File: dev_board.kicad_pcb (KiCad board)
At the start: 2 copper layers, 60 x 70 mm, 148 parts, among them IC1 AD9609BCPZRL7-80, IC2 ENS161-BLGT_LGA9_T&R_1k5, IC3 ICM-42670-P, IC4 IWRL6432BDBAAMFR, IC5 MP4541GN-Z, IC6 THS8136IPHPR, IC7 TPS40304ADRCR, IC8 XCC1352R1F3RGZR, J2 Conn_02x26_Odd_Even, J4 SM03B-SRSS-TB, J5 STM32H7 GPIO/Fabric Breakout A, J6 STM32H7 GPIO/Fabric Breakout B, J9 HS/IWRL Fabric Breakout, SW1 SW_Push, SW2 SW_Push, U1 RP2350_80QFN, U2 LPS22HH, U3 STM32H750VBTx, U4 LAN8742A, Y1 ABM8-272-T3

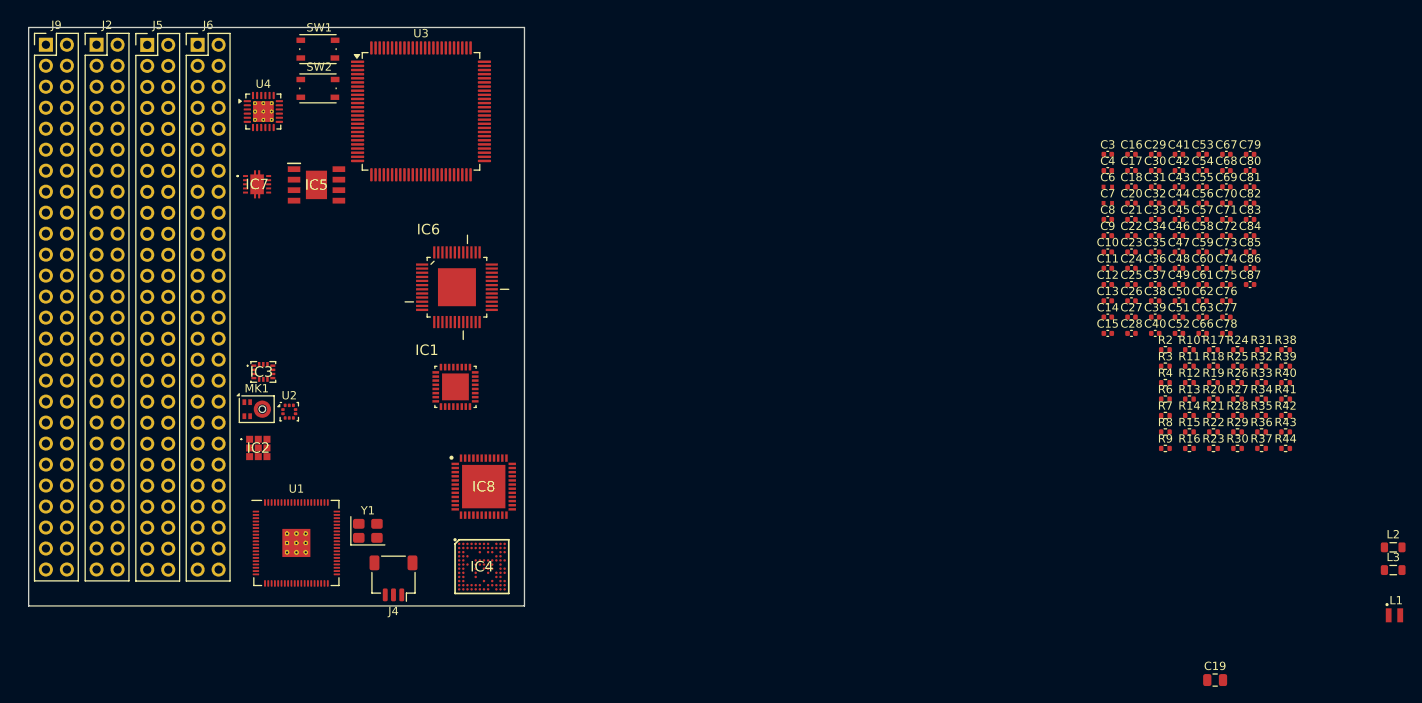
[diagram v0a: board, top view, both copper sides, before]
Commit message: more pcb chanegs, placements
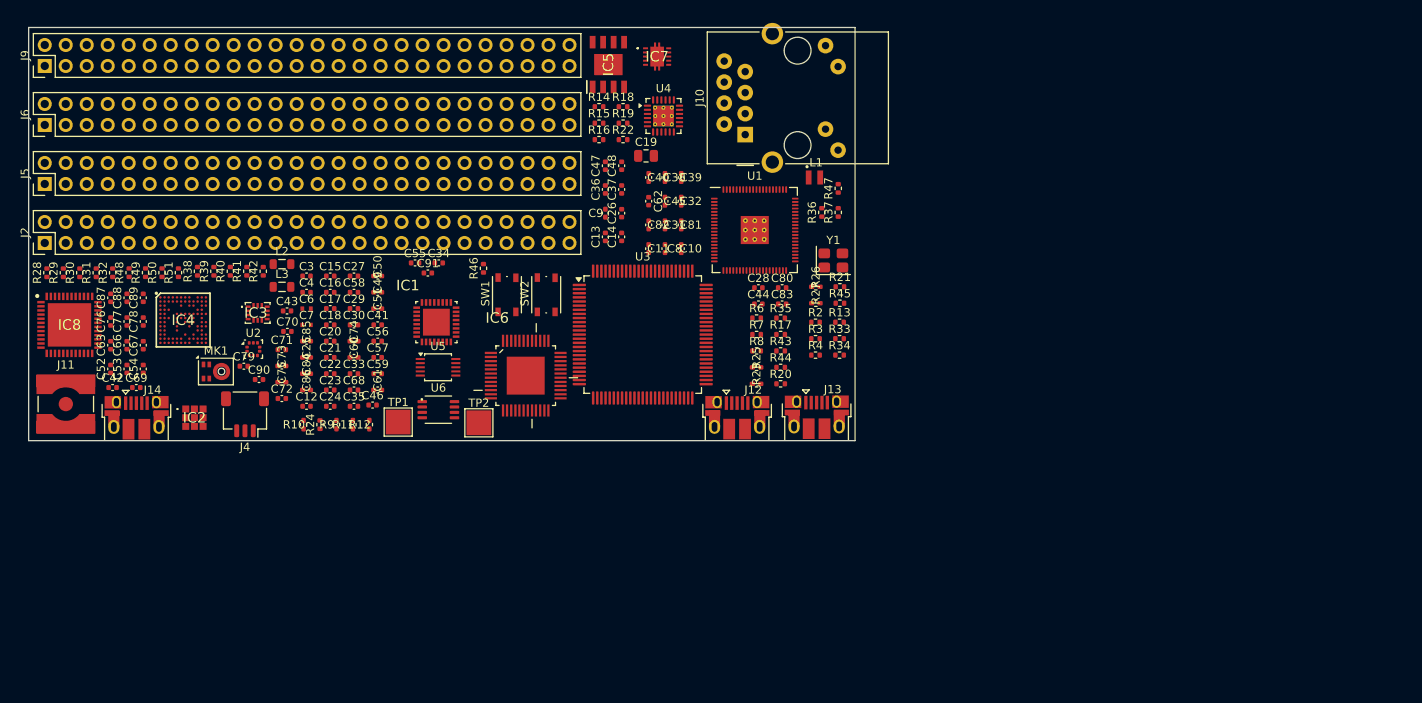
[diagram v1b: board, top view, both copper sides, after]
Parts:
- added C88: 100n, Capacitor_SMD:C_0402_1005Metric, F.Cu at (11.9, 32.7)
- added C89: 1n, Capacitor_SMD:C_0402_1005Metric, F.Cu at (13.9, 32.7)
- added C90: 100n, Capacitor_SMD:C_0402_1005Metric, F.Cu at (27.9, 42.6)
- added C91: 22p, Capacitor_SMD:C_0402_1005Metric, F.Cu at (48.3, 29.7)
- added J10: RJ45 / 8P8C LED, Connector_RJ:RJ45_Amphenol_RJMG1BD3B8K1ANR, F.Cu at (86.7, 13.0)
- added J11: SMA_RF_LAUNCH, Connector_Coaxial:SMA_Amphenol_132134-10_Vertical, F.Cu at (4.50, 45.6)
- added J12: RP2350 USB PROGRAM, Connector_USB:USB_Micro-B_Amphenol_10103594-0001LF_Horizontal, F.Cu at (85.8, 47.2)
- added J13: STM32 USB DFU ALT, Connector_USB:USB_Micro-B_Amphenol_10103594-0001LF_Horizontal, F.Cu at (95.4, 47.2)
- added J14: CC1352 PROG BRIDGE USB, Connector_USB:USB_Micro-B_Amphenol_10103594-0001LF_Horizontal, F.Cu at (13.1, 47.2)
- added R45: 1k, Resistor_SMD:R_0402_1005Metric, F.Cu at (98.2, 33.4)
- added R46: 1k, Resistor_SMD:R_0402_1005Metric, F.Cu at (55.0, 29.1)
- added R47: 1k, Resistor_SMD:R_0402_1005Metric, F.Cu at (98.0, 19.5)
- added R48: 1k, Resistor_SMD:R_0402_1005Metric, F.Cu at (12.2, 29.7)
- added R49: 33, Resistor_SMD:R_0402_1005Metric, F.Cu at (14.2, 29.7)
- added R50: 33, Resistor_SMD:R_0402_1005Metric, F.Cu at (16.1, 29.7)
- added R51: 0R/DNP, Resistor_SMD:R_0402_1005Metric, F.Cu at (18.1, 29.7)
- added TP1: TestPoint, TestPoint:TestPoint_Pad_3.0x3.0mm, F.Cu at (44.7, 47.8)
- added TP2: TestPoint, TestPoint:TestPoint_Pad_3.0x3.0mm, F.Cu at (54.5, 47.8)
- added U5: PGA113, Package_SO:TSSOP-10_3x3mm_P0.5mm, F.Cu at (49.5, 41.1)
- added U6: MCP6D11T-E/MS, MCP6D11T:MCP6D11T-E_MSOP-8_3x3mm_P0.65mm, F.Cu at (49.6, 46.2)
- moved R28 145.1 mm to (2.21, 29.7), turned to 90 degrees
- moved R29 143.4 mm to (4.20, 29.7), turned to 90 degrees
- moved R30 141.7 mm to (6.19, 29.7), turned to 90 degrees
- moved R31 141.3 mm to (8.18, 29.7), turned to 90 degrees
- moved R32 139.5 mm to (10.2, 29.7), turned to 90 degrees
- moved L2 138.8 mm to (30.7, 28.6)
- moved L3 138.8 mm to (30.7, 31.4)
- moved C87 137.9 mm to (9.93, 32.7), turned to 90 degrees
- moved C76 135.0 mm to (9.93, 35.6), turned to 90 degrees
- moved C69 134.1 mm to (13.0, 43.6)
- moved C67 133.1 mm to (13.9, 38.5), turned to 90 degrees
- moved C77 133.0 mm to (11.9, 35.6), turned to 90 degrees
- moved C53 132.7 mm to (11.9, 41.3), turned to 90 degrees
- moved C63 132.2 mm to (9.93, 38.5), turned to 90 degrees
- moved R38 132.0 mm to (20.4, 29.5), turned to 90 degrees
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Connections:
- net Net-(U1-USB_DM) renamed /CC_SPI_MISO
- net Net-(U1-USB_DP) renamed /CC_SPI_CS_N
- IC2 pad 2: /SENS_I2C_SCL -> unconnected-(IC2-SCLK_/_SCL-Pad2)
- IC2 pad 3: /ENS_ADDR -> unconnected-(IC2-MISO_/_ADDR-Pad3)
- IC2 pad 4: +3V3 -> unconnected-(IC2-VDD-Pad4)
- IC2 pad 5: +3V3 -> unconnected-(IC2-VDDIO-Pad5)
- IC2 pad 7: +3V3 -> unconnected-(IC2-CSN-Pad7)
- IC2 pad 8: GND -> unconnected-(IC2-VSS_1-Pad8)
- IC2 pad 9: GND -> unconnected-(IC2-VSS_2-Pad9)
- IC3 pad 4: /GPIO7 -> unconnected-(IC3-INT1_/_INT-Pad4)
- IC3 pad 5: +3V3 -> unconnected-(IC3-VDDIO-Pad5)
- IC3 pad 6: GND -> unconnected-(IC3-GND-Pad6)
- IC3 pad 7: /IMU_FSYNC -> unconnected-(IC3-FSYNC-Pad7)
- IC3 pad 9: /GPIO8 -> unconnected-(IC3-INT2-Pad9)
- IC8 pad 1: /CC_RF_P_2G4 -> unconnected-(IC8-RF_P_2_4GHZ-Pad1)
- IC8 pad 2: /CC_RF_N_2G4 -> unconnected-(IC8-RF_N_2_4GHZ-Pad2)
- IC8 pad 3: /CC_RF_P_SUBG -> unconnected-(IC8-RF_P_SUB_1GHZ-Pad3)
- IC8 pad 4: /CC_RF_N_SUBG -> unconnected-(IC8-RF_N_SUB_1GHZ-Pad4)
- IC8 pad 6: /CC_X32K_Q1 -> unconnected-(IC8-X32K_Q1-Pad6)
- IC8 pad 7: /CC_X32K_Q2 -> unconnected-(IC8-X32K_Q2-Pad7)
- MK1 pad 1: /GPIO3 -> GND
- MK1 pad 2: +3V3 -> GND
- MK1 pad 4: GND -> /GPIO3
- MK1 pad 5: GND -> +3V3
- U2 pad 1: +3V3 -> unconnected-(U2-Vdd_IO-Pad1)
- U2 pad 10: +3V3 -> unconnected-(U2-VDD-Pad10)
- U2 pad 2: /SENS_I2C_SCL -> unconnected-(U2-SCL-Pad2)
- U2 pad 3: GND -> +3V3
- U2 pad 4: /SENS_I2C_SDA -> unconnected-(U2-SDA-Pad4)
- U2 pad 5: /LPS_SA0 -> /GPIO9
- U2 pad 7: /GPIO9 -> /LPS_SA0
- U2 pad 8: GND -> +3V3
- U2 pad 9: GND -> +3V3
- U3 pad 12: /GPIO37 -> /STM_VCAP_A
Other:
- board size 60 x 70 mm -> 100 x 50 mm
- copper layers 2 -> 4
